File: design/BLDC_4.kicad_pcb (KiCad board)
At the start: 4 copper layers, 103 x 63 mm, 233 parts, among them K1 SERVO, P1 CANBUS, P10 MOTOR3, P11 MOTOR2, P12 MOTOR1, P13 SWD, P14 IN+, P15 PWR_COMM_2, P2 HALL/Encoder, P3 HALL/Encoder, P4 PWR_COMM_1, P5 IN+, P6 IN-, P7 MOTOR3, P8 MOTOR2, P9 MOTOR1, Q1 FDBL0630N150, Q10 FDBL0630N150, Q11 FDBL0630N150, Q12 FDBL0630N150, Q2 FDBL0630N150, Q3 FDBL0630N150, Q4 FDBL0630N150, Q5 FDBL0630N150, Q6 FDBL0630N150, Q7 FDBL0630N150, Q8 FDBL0630N150, Q9 FDBL0630N150, U1 SN65HVD232, U2 DRV8302, U3 NCP1117ST33T3G, U4 STM32F40X_LQFP144, U5 DRV8302, U6 NCP1117ST33T3G, X1 MINI-USB-SHIELD-32005-201, X2 8MHz 10ppm

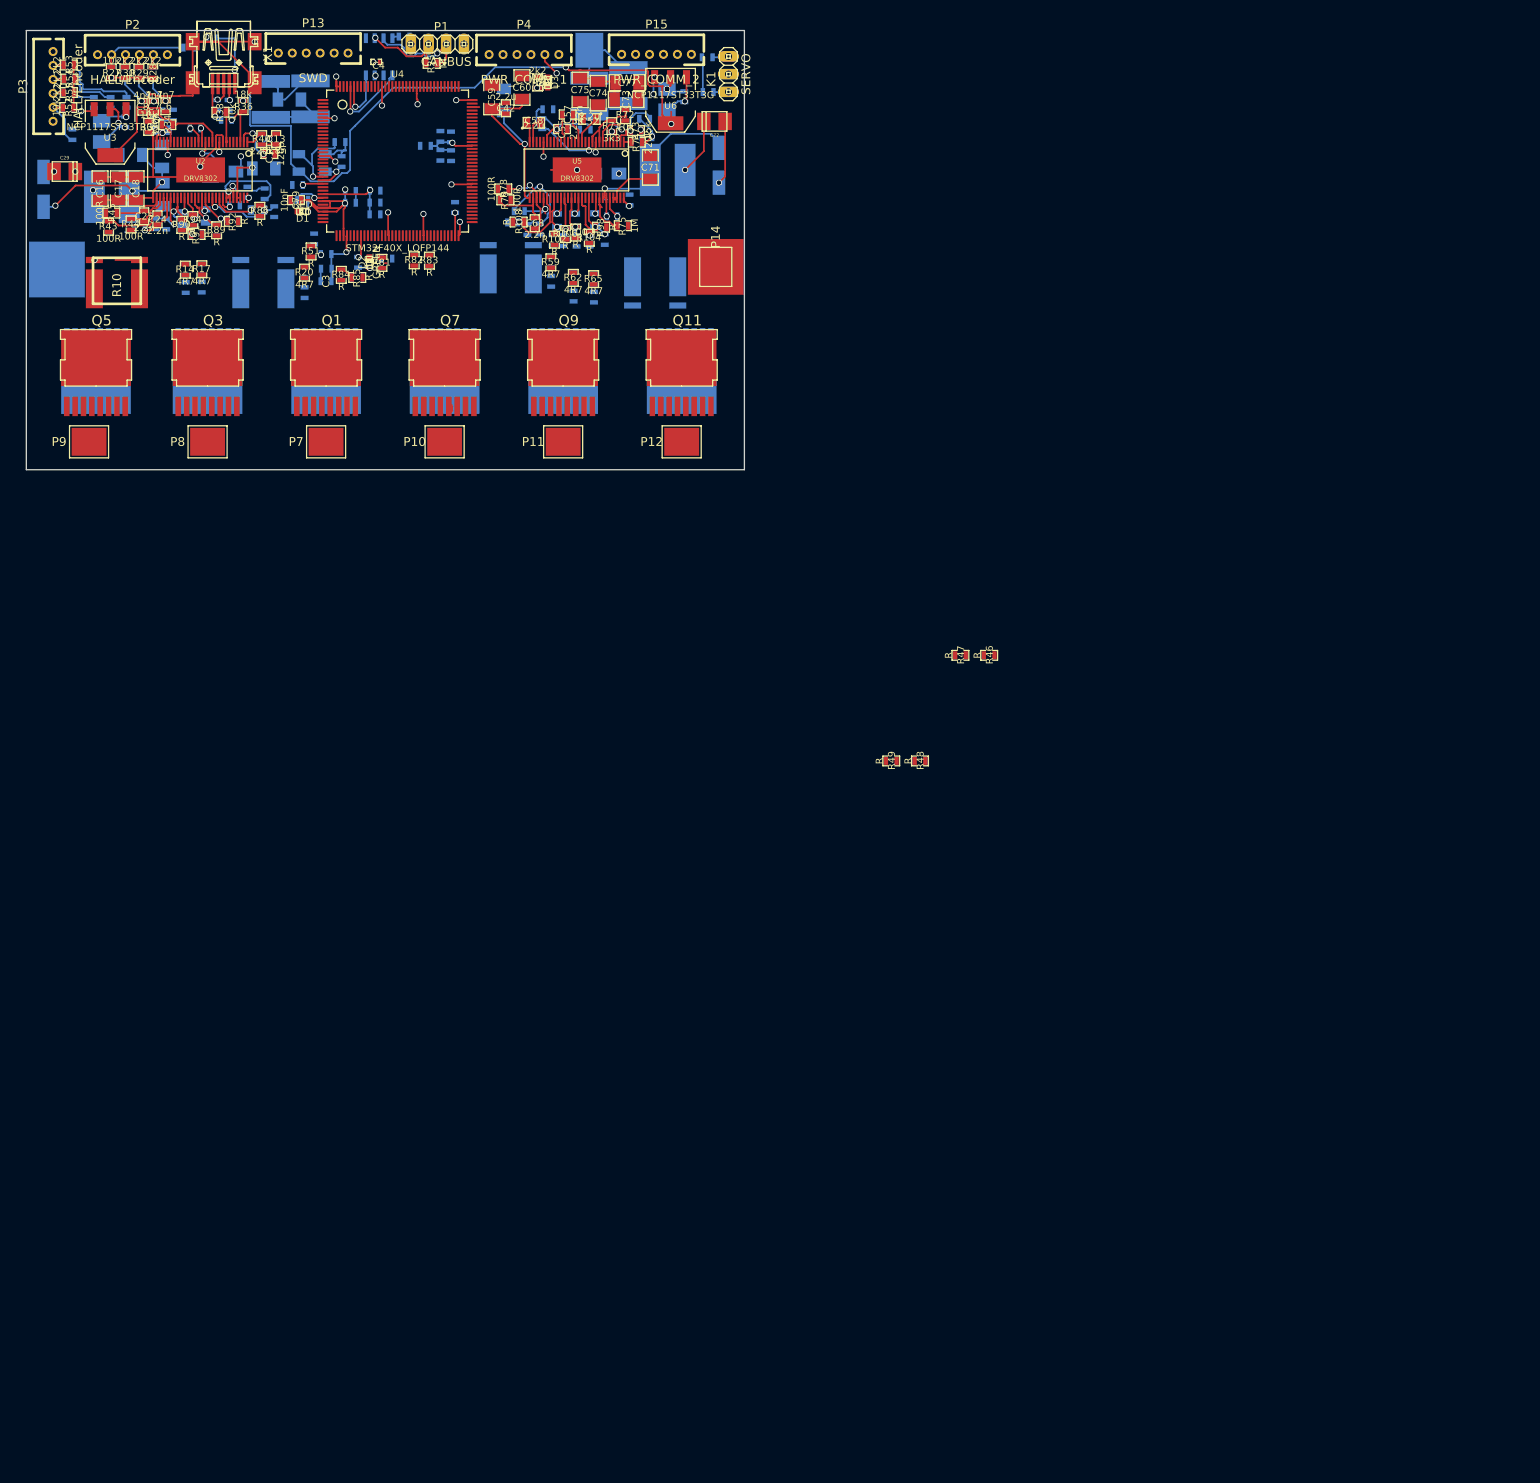
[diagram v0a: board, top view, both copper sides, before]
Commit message: New pcb layout
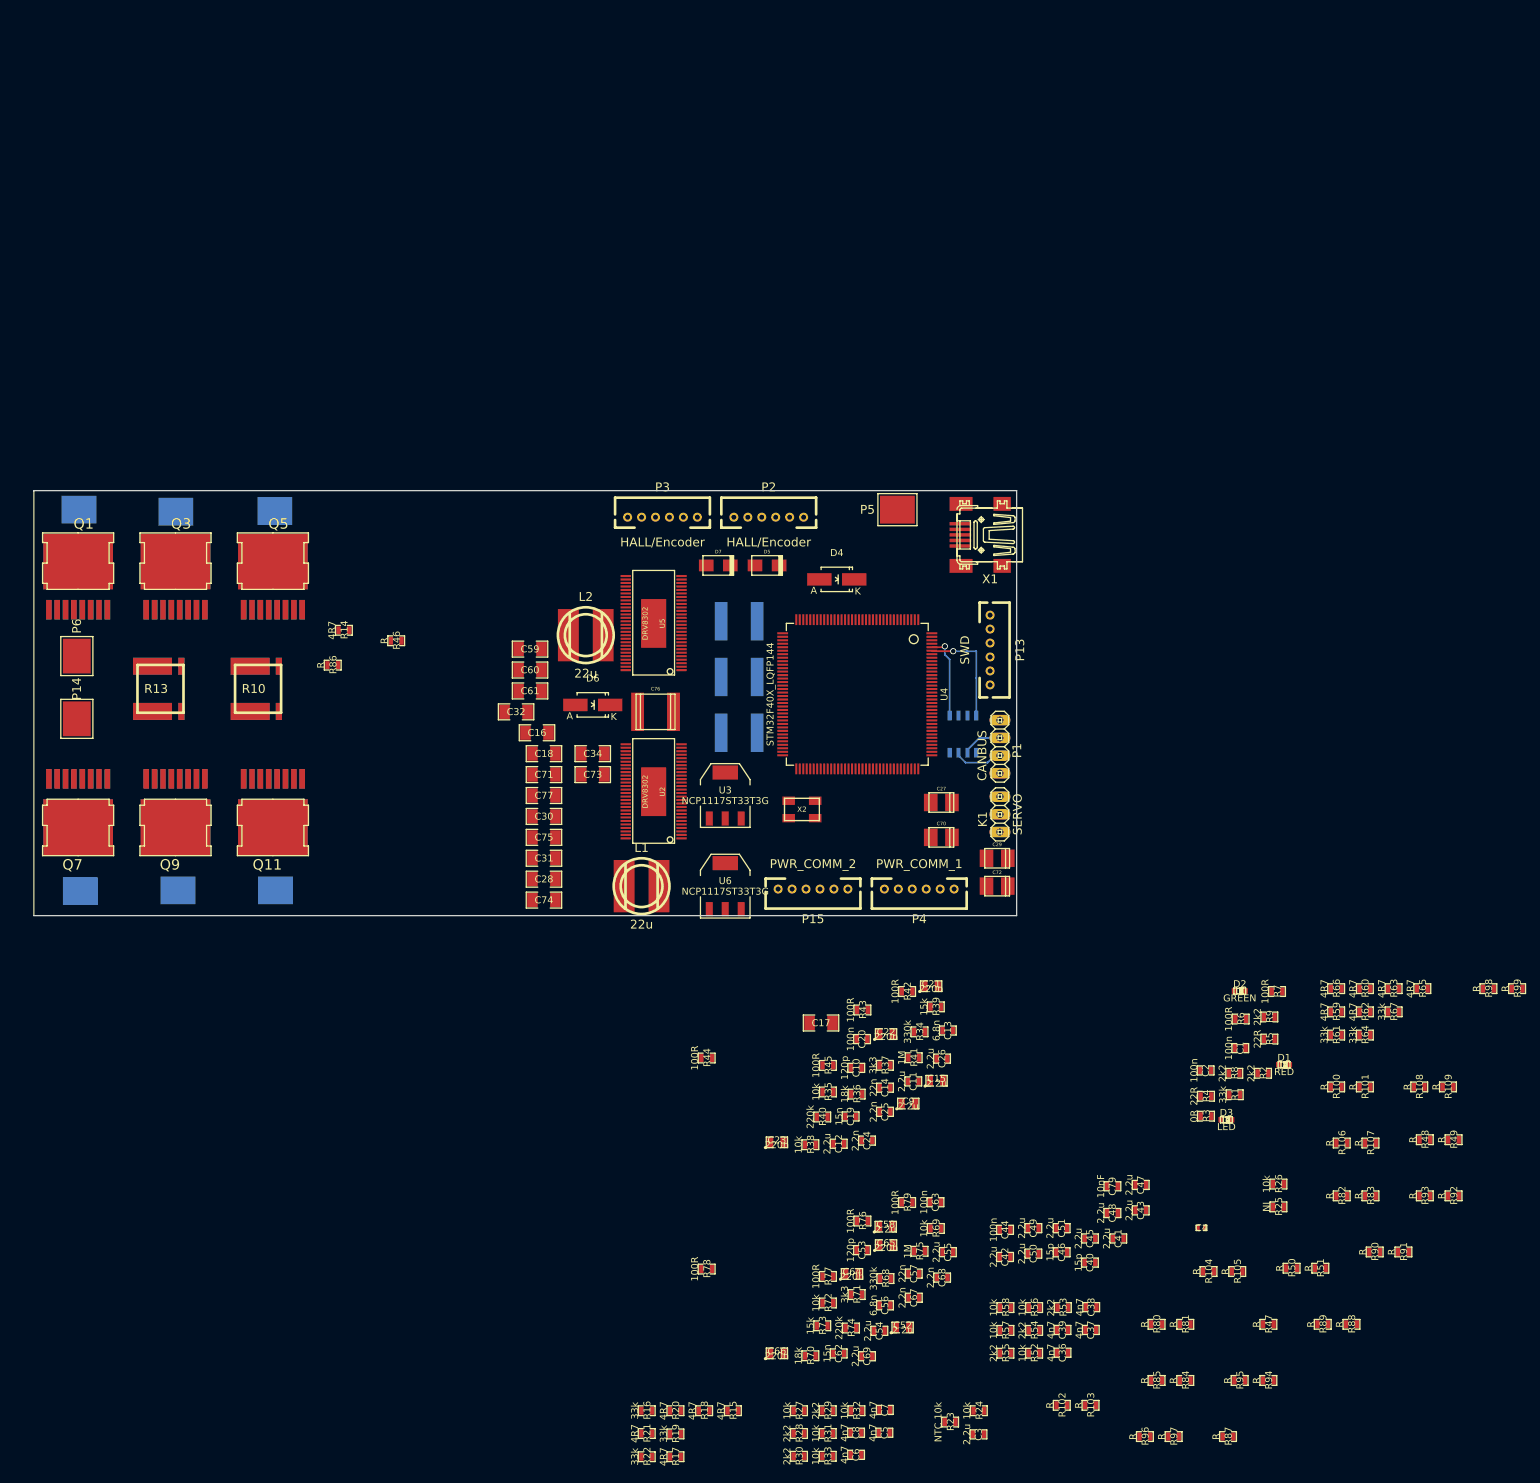
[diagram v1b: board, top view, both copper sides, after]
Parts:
- C1, C11, C12, C14, C15, C19, C2, C20, C21, C22, C23, C26, C27, C28, C3, C30, C31, C32, C34, C36, C37, C38, C39, C40, C41, C43, C44, C45, C46, C47, C48, C49, C5, C50, C51, C53, C54, C56, C61, C62, C63, C64, C65, C66, C67, C69, C70, C76, C9, D4, D5, D6, D7, L1, L2, P5, P6, R1, R101, R103, R105, R107, R109, R13, R15, R16, R18, R19, R2, R21, R22, R23, R24, R26, R3, R31, R32, R33, R37, R39, R4, R41, R42, R5, R50, R56, R57, R58, R6, R60, R61, R63, R64, R66, R67, R68, R69, R7, R70, R76, R77, R80, R87, R88, R9, R93, R95, R96, R97, R99, X2: moved to F.Cu
- P10, P11, P12, P7, P8, P9: moved to B.Cu
- moved R53 228.2 mm to (184.4, 245.5)
- moved R97 227.1 mm to (200.3, 264.0), turned to 0 degrees
- moved R94 226.9 mm to (213.9, 255.9), turned to 0 degrees
- moved R54 226.6 mm to (180.3, 248.7)
- moved R91 226.4 mm to (233.3, 237.5), turned to 0 degrees
- moved R52 226.1 mm to (180.3, 252.0)
- moved R88 226.0 mm to (225.8, 247.9), turned to 0 degrees
- moved R90 225.8 mm to (229.2, 237.5), turned to 0 degrees
- moved R56 225.7 mm to (180.3, 245.5)
- moved R55 225.3 mm to (176.2, 252.0)
- moved C36 225.2 mm to (184.4, 251.9), turned to 0 degrees
- moved C39 224.3 mm to (184.4, 248.7), turned to 0 degrees
- moved R57 224.2 mm to (176.2, 248.7)
- moved R92 224.0 mm to (240.5, 229.4), turned to 0 degrees
- moved R95 223.9 mm to (209.8, 255.9), turned to 0 degrees
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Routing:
- net VCC: track 305.2 -> 0.00 mm, vias 27 -> 0
- net +5V: track 193.3 -> 0.00 mm, vias 11 -> 0
- net (no net): track 145.4 -> 0.00 mm, vias 3 -> 0
- net GND: track 118.0 -> 0.00 mm, vias 9 -> 0
- net V_SUPPLY: track 86.8 -> 0.00 mm, vias 3 -> 0
- net /Mosfet driver/Voltage_divider.sch/OUT: track 47.3 -> 0.00 mm, vias 8 -> 0
- net /Mosfet driver_2/Voltage_divider.sch/OUT: track 41.1 -> 0.00 mm, vias 7 -> 0
- net Net-(C20-Pad1): track 40.1 -> 0.00 mm, vias 3 -> 0
- net Net-(C63-Pad1): track 28.2 -> 0.00 mm, vias 2 -> 0
- net Net-(R34-Pad2): track 14.8 -> 0.00 mm
- net Net-(C67-Pad2): track 13.7 -> 0.00 mm, vias 1 -> 0
- net Net-(R68-Pad2): track 13.2 -> 0.00 mm, vias 1 -> 0
- net /Filters/TEMP_IN: track 12.5 -> 0.00 mm
- net Net-(C40-Pad1): track 11.7 -> 0.00 mm, vias 1 -> 0
- net Net-(C24-Pad2): track 11.3 -> 0.00 mm
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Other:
- board size 103 x 63 mm -> 141 x 61 mm
